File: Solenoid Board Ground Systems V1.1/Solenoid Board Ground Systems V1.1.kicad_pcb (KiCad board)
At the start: 2 copper layers, 63.5 x 33 mm, 27 parts, among them J1 OUT CHAN A, J2 POWER IN, J3 OUT CHAN B

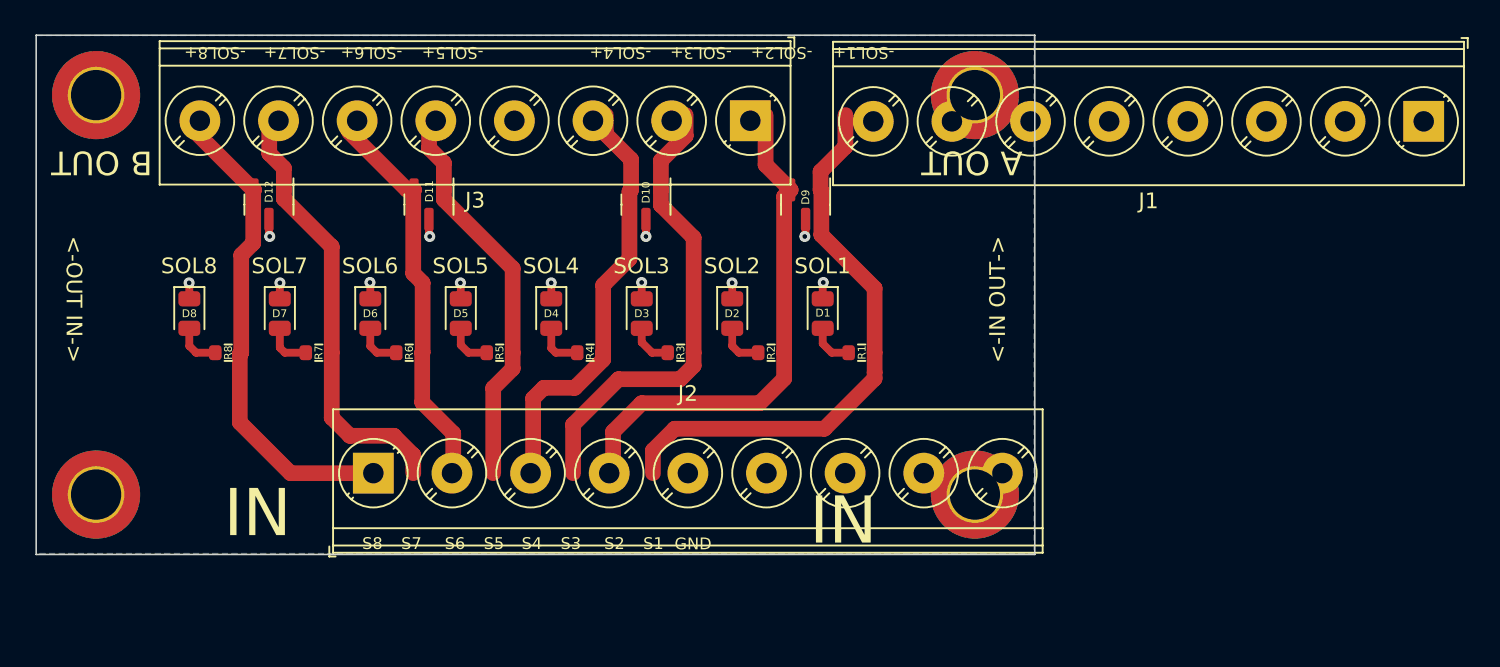
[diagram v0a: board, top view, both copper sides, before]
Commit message: Revions and new board
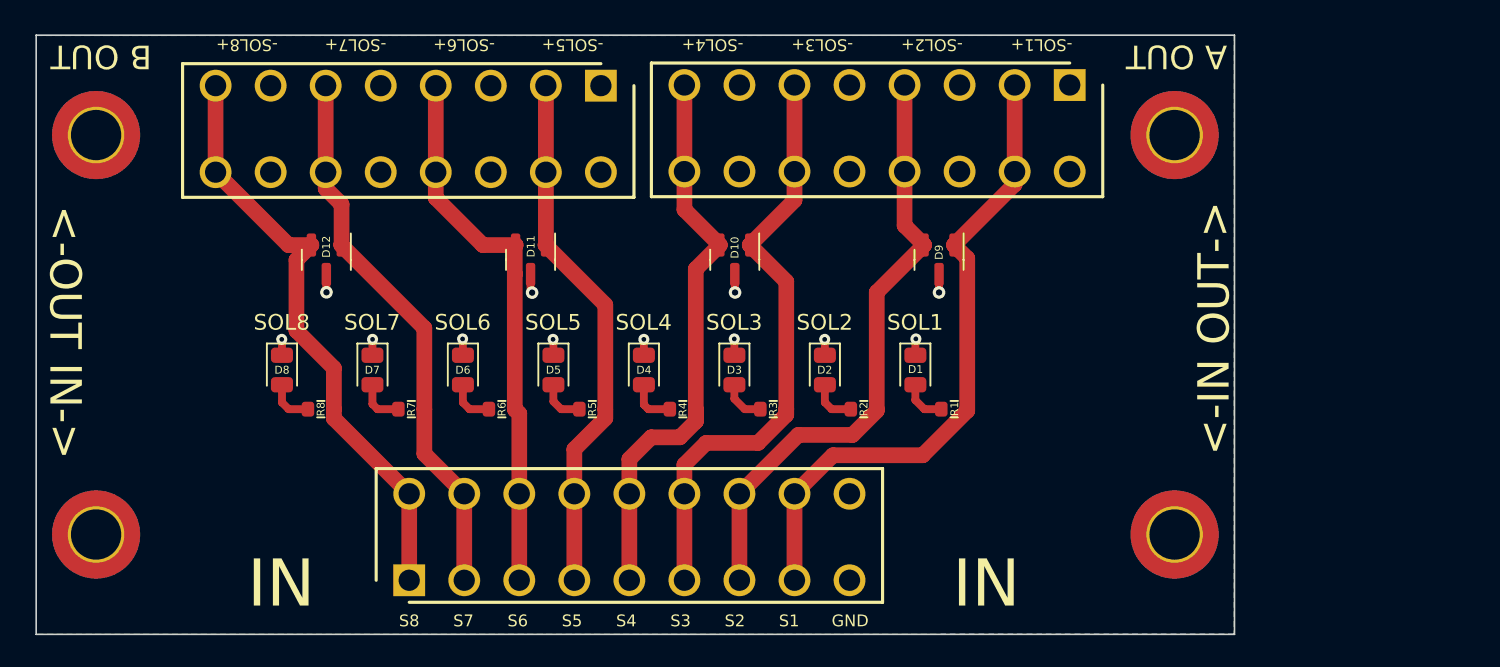
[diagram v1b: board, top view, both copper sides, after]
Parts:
- J1: value OUT CHAN A -> TBLH10V-350-09BK; footprint TerminalBlock_Phoenix:TerminalBlock_Phoenix_PT-1,5-8-5.0-H_1x08_P5.00mm_Horizontal -> TBLH10V-350-09BK:RHDR18W80P550X350_2X9_3220X850X1420P
- J2: value POWER IN -> TBLH10V-350-08BK; footprint TerminalBlock_Phoenix:TerminalBlock_Phoenix_PT-1,5-9-5.0-H_1x09_P5.00mm_Horizontal -> TBLH10V-350-08BK:RHDR16W80P550X350_2X8_2870X850X1420P
- J3: value OUT CHAN B -> TBLH10V-350-08BK; footprint TerminalBlock_Phoenix:TerminalBlock_Phoenix_PT-1,5-8-5.0-H_1x08_P5.00mm_Horizontal -> TBLH10V-350-08BK:RHDR16W80P550X350_2X8_2870X850X1420P
- moved J1 70.8 mm to (49.1, 60.1), turned to 0 degrees
- moved J2 50.7 mm to (91.1, 28.6), turned to 180 degrees
- moved H3 13.0 mm to (97.8, 31.8)
- moved H4 13.0 mm to (97.8, 57.1)
- moved J3 9.76 mm to (61.3, 28.6)
- moved D9 9.18 mm to (82.8, 39.7)
- moved D11 7.35 mm to (56.8, 39.7)
- moved D1 6.90 mm to (81.3, 46.7)
- moved D2 6.90 mm to (75.6, 46.7)
- moved D4 6.90 mm to (64.0, 46.7)
- moved D5 6.90 mm to (58.3, 46.7)
- moved D6 6.90 mm to (52.5, 46.7)
- moved D7 6.90 mm to (46.8, 46.7)
- moved R1 6.90 mm to (83.8, 49.2)
- moved R2 6.90 mm to (78.0, 49.2)
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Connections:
- J1 pad 1: GND -> POW IN H
- J1 pad 2: POW IN A -> POW IN H
- J1 pad 3: GND -> POW IN G
- J1 pad 4: POW IN B -> POW IN G
- J1 pad 5: GND -> POW IN F
- J1 pad 6: POW IN C -> POW IN F
- J1 pad 7: GND -> POW IN E
- J1 pad 8: POW IN D -> POW IN E
- J2 pad 1: POW IN H -> GND
- J2 pad 2: POW IN G -> GND
- J2 pad 3: POW IN F -> POW IN A
- J2 pad 4: POW IN E -> POW IN A
- J2 pad 5: POW IN D -> GND
- J2 pad 6: POW IN C -> GND
- J2 pad 8: POW IN A -> POW IN B
- J3 pad 2: POW IN E -> GND
- J3 pad 3: GND -> POW IN E
- J3 pad 4: POW IN F -> POW IN E
- J3 pad 6: POW IN G -> GND
- J3 pad 7: GND -> POW IN F
- J3 pad 8: POW IN H -> POW IN F
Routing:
- net POW IN D: track 27.2 -> 36.6 mm
- net POW IN F: track 25.8 -> 34.9 mm
- net POW IN C: track 29.8 -> 38.2 mm
- net POW IN E: track 25.5 -> 33.9 mm
- net POW IN G: track 28.2 -> 35.1 mm
- net POW IN H: track 31.5 -> 38.2 mm
- net POW IN B: track 32.5 -> 38.9 mm
- net POW IN A: track 36.3 -> 41.3 mm
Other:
- board size 63.5 x 33 mm -> 76.2 x 38.1 mm
